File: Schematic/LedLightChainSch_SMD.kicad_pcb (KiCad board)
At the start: 2 copper layers, 35.6 x 17.8 mm, 13 parts, among them J1 Led-Chain, J2 Out+, J3 Out-, J4 Batt+, J5 Batt-, J6 SWDIO, J7 TX, J8 Battery, Q1 BC817, SW1 SW_SPDT, U1 CH32V003JxMx

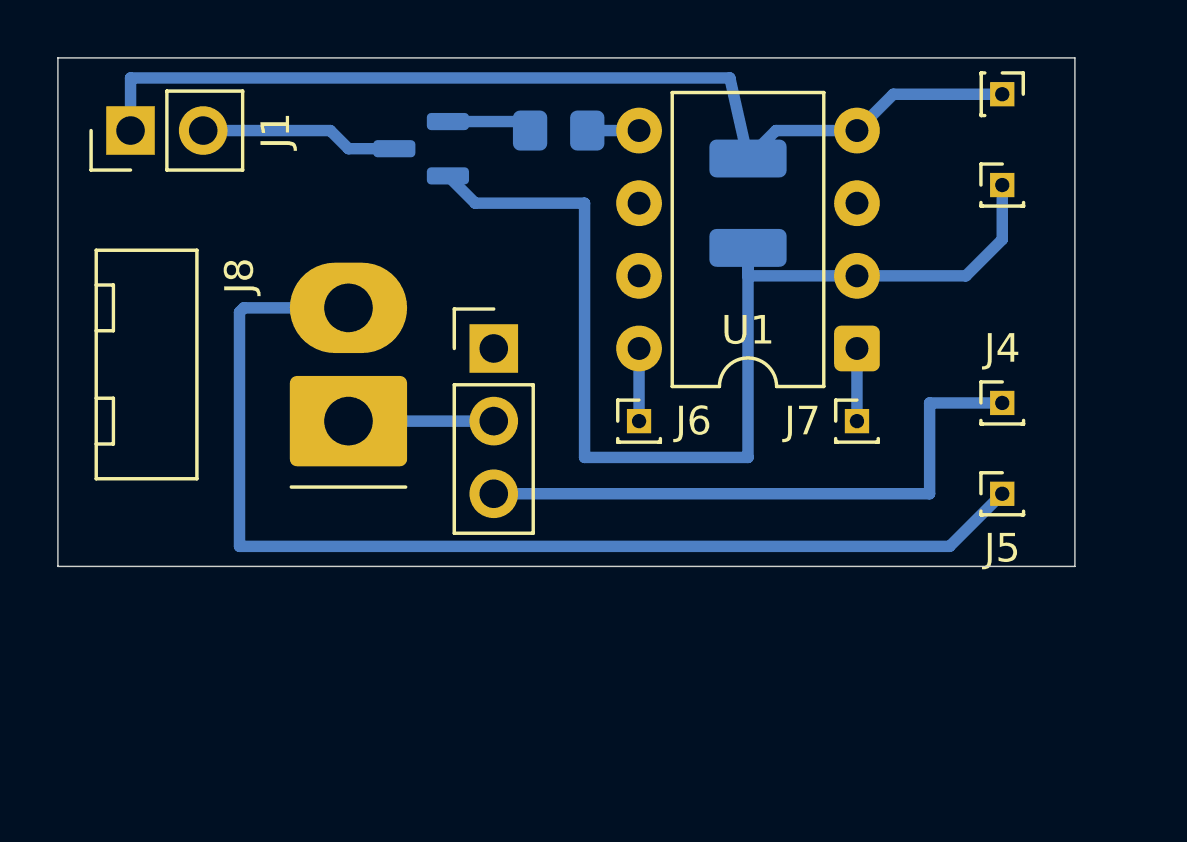
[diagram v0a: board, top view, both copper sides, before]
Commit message: Release with target hardware
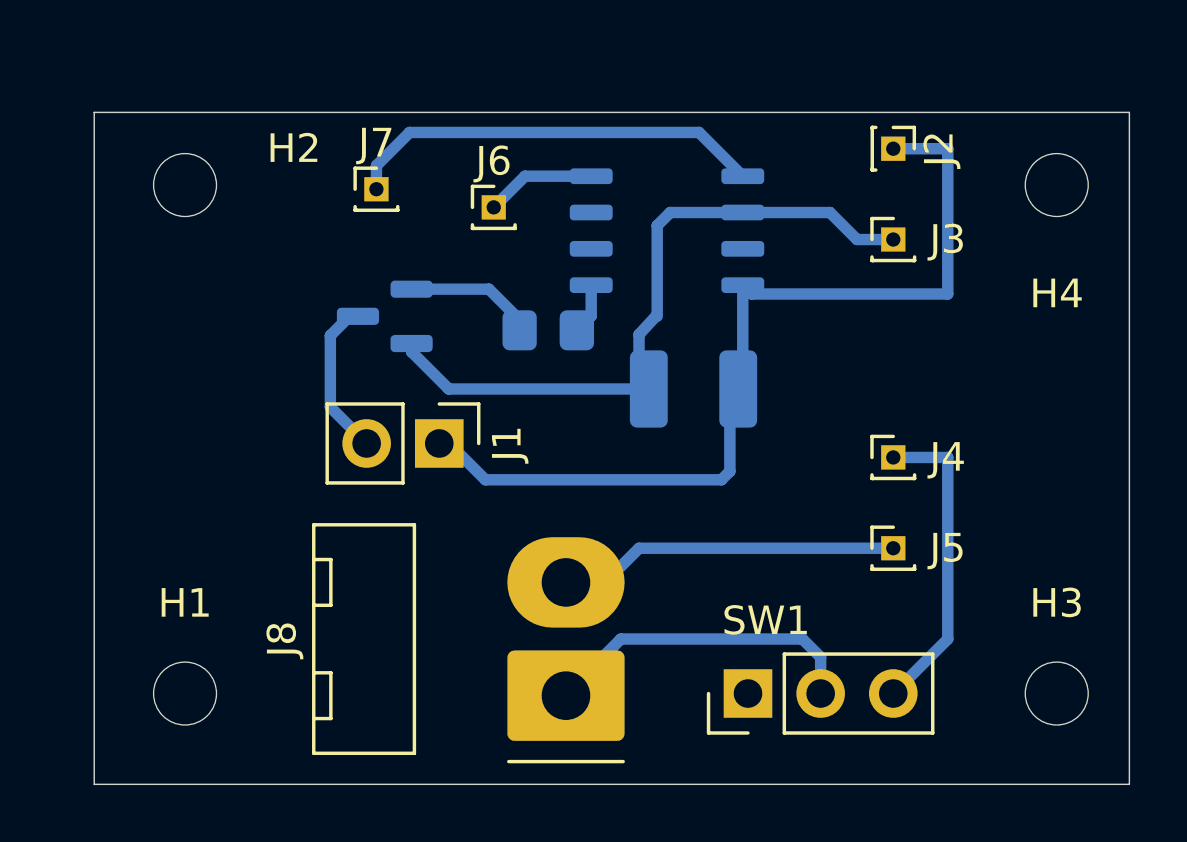
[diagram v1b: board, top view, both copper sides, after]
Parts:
- added H1: MountingHole, MountingHole:MountingHole_2.2mm_M2, F.Cu at (118.7, 113.7)
- added H2: MountingHole, MountingHole:MountingHole_2.2mm_M2, F.Cu at (118.7, 95.9)
- added H3: MountingHole, MountingHole:MountingHole_2.2mm_M2, F.Cu at (149.2, 113.7)
- added H4: MountingHole, MountingHole:MountingHole_2.2mm_M2, F.Cu at (149.2, 95.9)
- U1: footprint Package_DIP:DIP-8_W7.62mm -> Package_SO:JEITA_SOIC-8_3.9x4.9mm_P1.27mm; moved to B.Cu
- moved J7 18.7 mm to (125.4, 96.0)
- moved J1 15.4 mm to (127.6, 104.9), turned to -90 degrees
- moved SW1 15.0 mm to (138.4, 113.7), turned to 90 degrees
- moved J8 12.2 mm to (132.1, 113.7)
- moved J6 9.04 mm to (129.5, 96.7)
- moved U1 7.82 mm to (135.6, 97.5)
- moved R1 6.99 mm to (131.4, 101.0)
- moved C1 6.77 mm to (136.5, 103.0), turned to 180 degrees
- moved Q1 6.00 mm to (125.7, 100.5)
- moved J2 4.26 mm to (143.5, 94.6)
- moved J3 4.26 mm to (143.5, 97.8)
- moved J4 4.26 mm to (143.5, 105.4)
- moved J5 4.26 mm to (143.5, 108.6)
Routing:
- net Net-(J5-Pin_1): track 39.5 -> 11.9 mm
- net GND: track 39.4 -> 23.9 mm
- net Net-(J7-Pin_1): track 2.54 -> 14.7 mm
- net Net-(J4-Pin_1): track 21.0 -> 10.9 mm
- net Net-(J8-Pin_1): track 5.08 -> 11.2 mm
- net +4V: track 35.5 -> 32.0 mm
- net Net-(Q1-B): track 3.00 -> 4.59 mm
- net Net-(J1-Pin_2): track 6.95 -> 5.54 mm
- net Net-(J6-Pin_1): track 2.54 -> 3.86 mm
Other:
- board size 35.6 x 17.8 mm -> 36.2 x 23.5 mm
